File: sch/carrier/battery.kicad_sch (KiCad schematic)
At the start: 9 parts

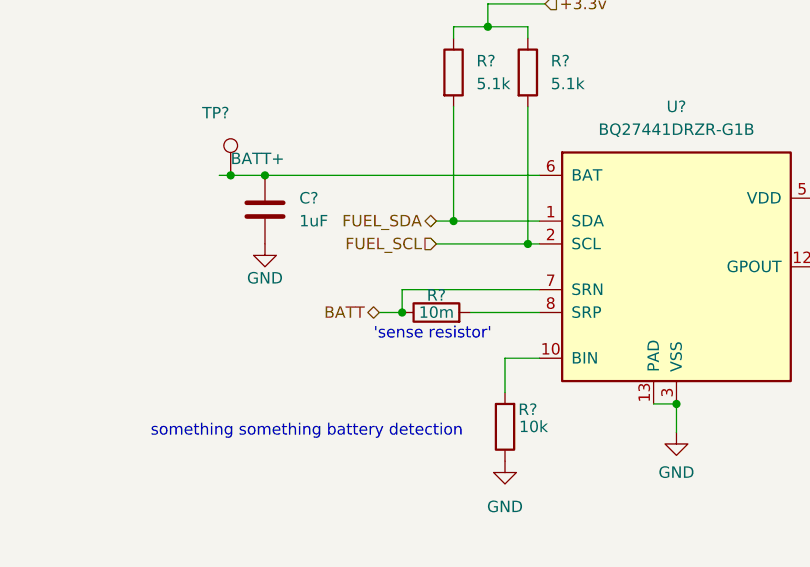
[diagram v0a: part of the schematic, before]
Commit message: we're abt ready to do pcb i hope!
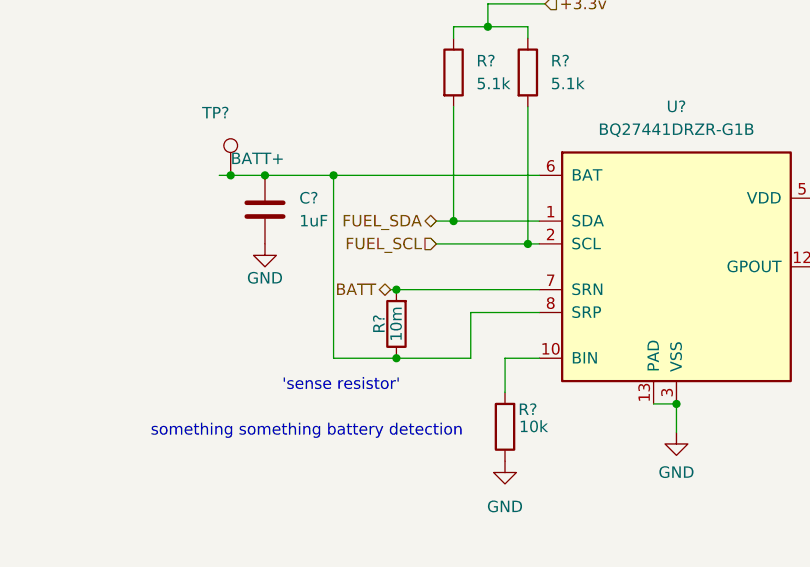
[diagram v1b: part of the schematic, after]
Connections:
- net BATT: now also R?.2; no longer R?.1
- net at C?.1, TP?.1, U?.6 (BAT): now also R?.1, U?.8 (SRP)
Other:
- moved on the sheet: R?
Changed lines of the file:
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@@
   (junction (at 92.075 72.39) (diameter 0.9144) (color 0 0 0 0))
   (junction (at 95.885 72.39) (diameter 0.9144) (color 0 0 0 0))
-  (junction (at 111.125 87.63) (diameter 0.9144) (color 0 0 0 0))
+  (junction (at 103.505 72.39) (diameter 0.9144) (color 0 0 0 0))
+  (junction (at 110.49 85.09) (diameter 0.9144) (color 0 0 0 0))
+  (junction (at 110.49 92.71) (diameter 0.9144) (color 0 0 0 0))
   (junction (at 116.84 77.47) (diameter 0.9144) (color 0 0 0 0))
   (junction (at 120.65 55.88) (diameter 0.9144) (color 0 0 0 0))
@@
     (stroke (width 0) (type solid) (color 0 0 0 0))
   )
-  (wire (pts (xy 95.885 72.39) (xy 126.365 72.39))
-    (stroke (width 0) (type solid) (color 0 0 0 0))
-  )
-  (wire (pts (xy 108.585 87.63) (xy 111.125 87.63))
-    (stroke (width 0) (type solid) (color 0 0 0 0))
-  )
-  (wire (pts (xy 111.125 85.09) (xy 111.125 87.63))
+  (wire (pts (xy 95.885 72.39) (xy 103.505 72.39))
+    (stroke (width 0) (type solid) (color 0 0 0 0))
+  )
+  (wire (pts (xy 103.505 72.39) (xy 126.365 72.39))
+    (stroke (width 0) (type solid) (color 0 0 0 0))
+  )
+  (wire (pts (xy 103.505 92.71) (xy 103.505 72.39))
+    (stroke (width 0) (type solid) (color 0 0 0 0))
+  )
+  (wire (pts (xy 109.855 85.09) (xy 110.49 85.09))
+    (stroke (width 0) (type solid) (color 0 0 0 0))
+  )
+  (wire (pts (xy 110.49 85.09) (xy 126.365 85.09))
+    (stroke (width 0) (type solid) (color 0 0 0 0))
+  )
+  (wire (pts (xy 110.49 92.71) (xy 103.505 92.71))
     (stroke (width 0) (type solid) (color 0 0 0 0))
   )
@@
     (stroke (width 0) (type solid) (color 0 0 0 0))
   )
-  (wire (pts (xy 118.745 87.63) (xy 126.365 87.63))
+  (wire (pts (xy 118.745 87.63) (xy 118.745 92.71))
+    (stroke (width 0) (type solid) (color 0 0 0 0))
+  )
+  (wire (pts (xy 118.745 92.71) (xy 110.49 92.71))
     (stroke (width 0) (type solid) (color 0 0 0 0))
   )
@@
     (stroke (width 0) (type solid) (color 0 0 0 0))
   )
-  (wire (pts (xy 126.365 85.09) (xy 111.125 85.09))
+  (wire (pts (xy 126.365 87.63) (xy 118.745 87.63))
     (stroke (width 0) (type solid) (color 0 0 0 0))
   )
@@
     (effects (font (size 1.27 1.27)) (justify left bottom))
   )
-  (text "'sense resistor'" (at 107.95 90.805 0)
+  (text "'sense resistor'" (at 97.79 96.52 0)
     (effects (font (size 1.27 1.27)) (justify left bottom))
   )
-  (hierarchical_label "BATT" (shape bidirectional) (at 108.585 87.63 180)
+  (hierarchical_label "BATT" (shape bidirectional) (at 109.855 85.09 180)
     (effects (font (size 1.27 1.27)) (justify right))
   )
@@
     (pin "1")
   )
-  (symbol (lib_id "Device:R") (at 114.935 87.63 90) (unit 1)
+  (symbol (lib_id "Device:R") (at 110.49 88.9 180) (unit 1)
     (in_bom yes) (on_board yes)
-    (property "Reference" "R?" (id 0) (at 114.935 85.725 90))
-    (property "Value" "10m" (id 1) (at 114.935 87.63 90))
-    (property "Footprint" "" (id 2) (at 114.935 89.408 90)
-      (effects (font (size 1.27 1.27)) hide)
-    )
-    (property "Datasheet" "~" (id 3) (at 114.935 87.63 0)
-      (effects (font (size 1.27 1.27)) hide)
-    )
+    (property "Reference" "R?" (id 0) (at 108.585 88.9 90))
+    (property "Value" "10m" (id 1) (at 110.49 88.9 90))
+    (property "Footprint" "" (id 2) (at 112.268 88.9 90)
+      (effects (font (size 1.27 1.27)) hide)
+    )
+    (property "Datasheet" "~" (id 3) (at 110.49 88.9 0)
+      (effects (font (size 1.27 1.27)) hide)
+    )
